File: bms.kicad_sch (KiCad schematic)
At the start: 146 parts, among them J1 Conn_01x08, Q1 DMZ6012E, Q2 DMZ6012E, Q5 BSS123, U8 XC6206P332MR, U9 2SC2383_C41375137

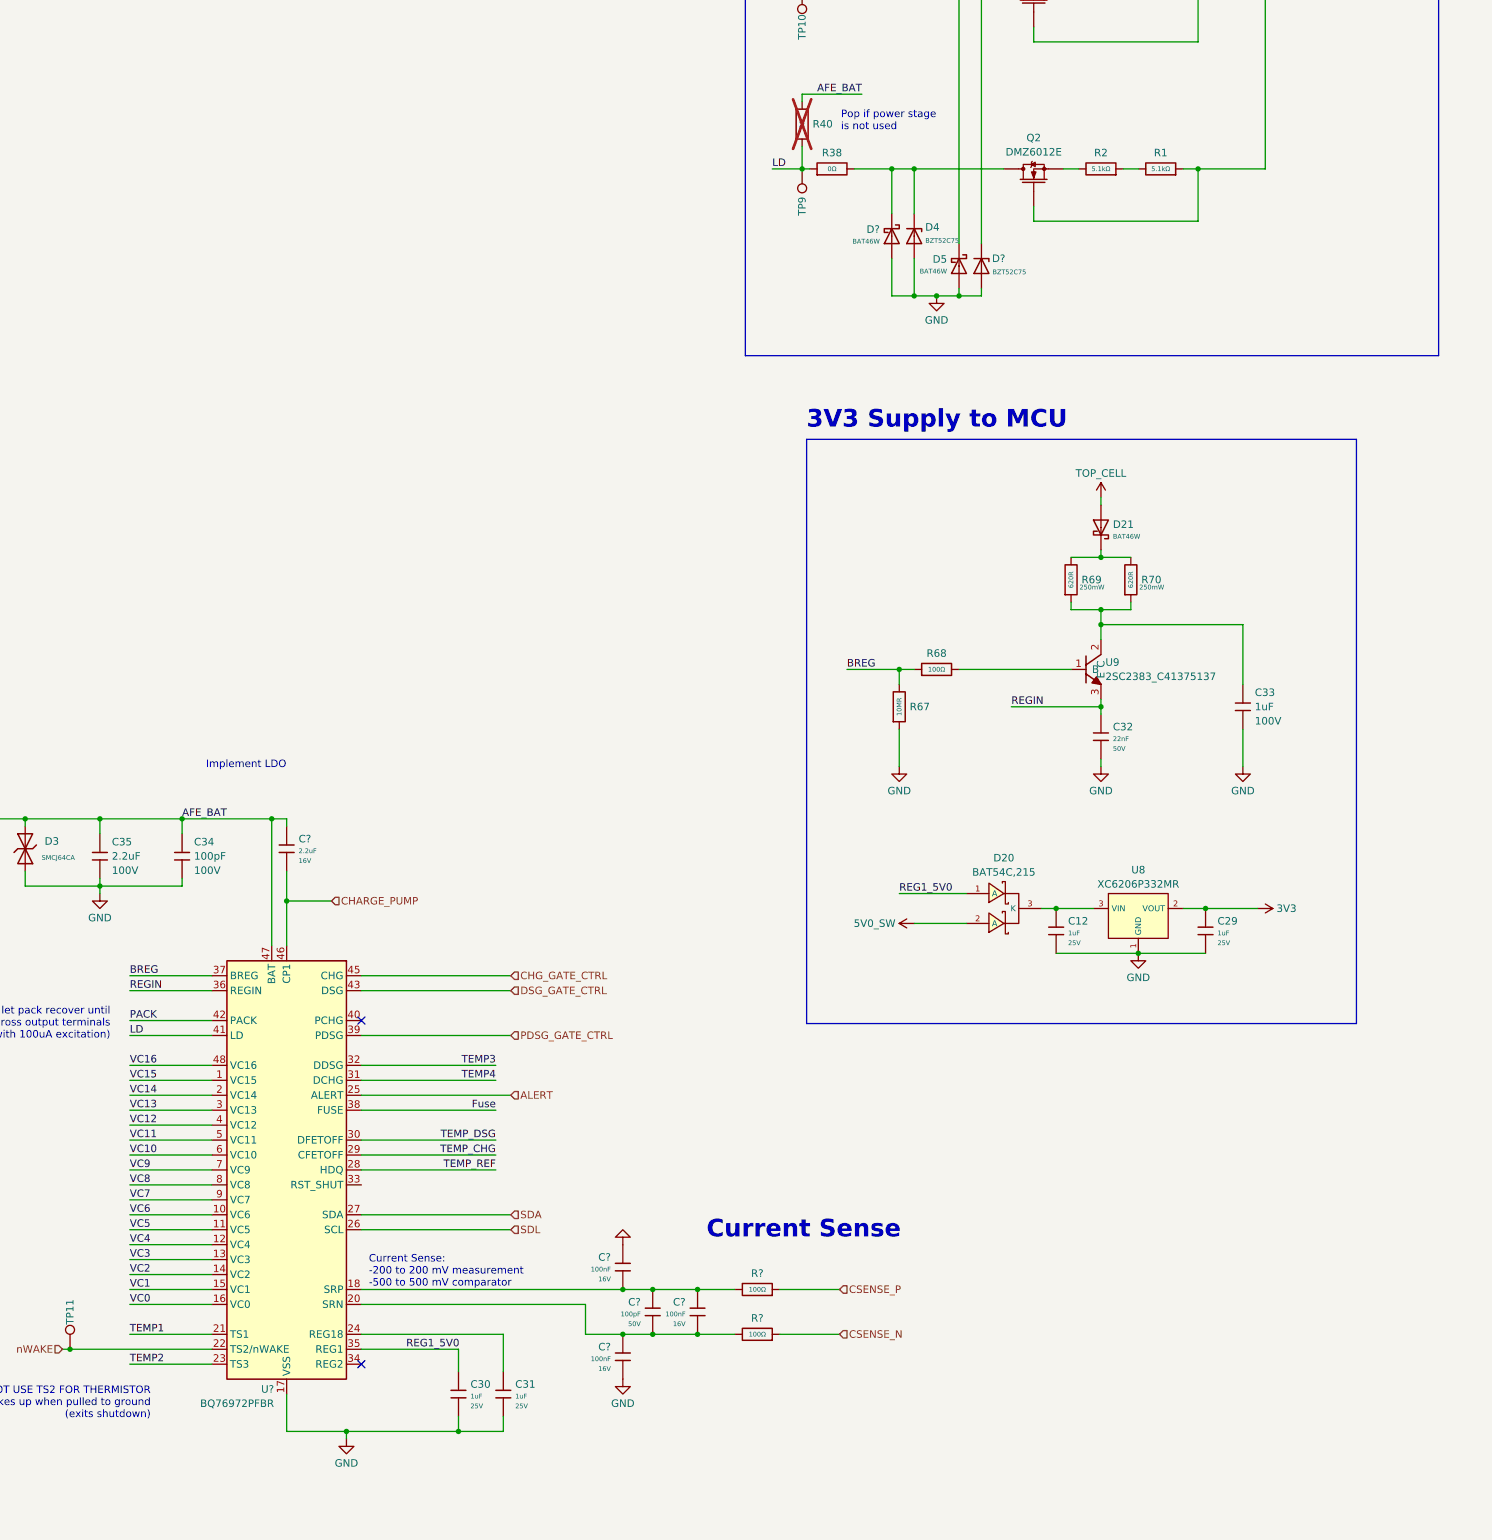
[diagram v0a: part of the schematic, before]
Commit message: Revert "added precharge circuit, filled in placeholder parts"
This reverts commit caa5444a50fe9d2ccb2e95970e40619801e9f697.
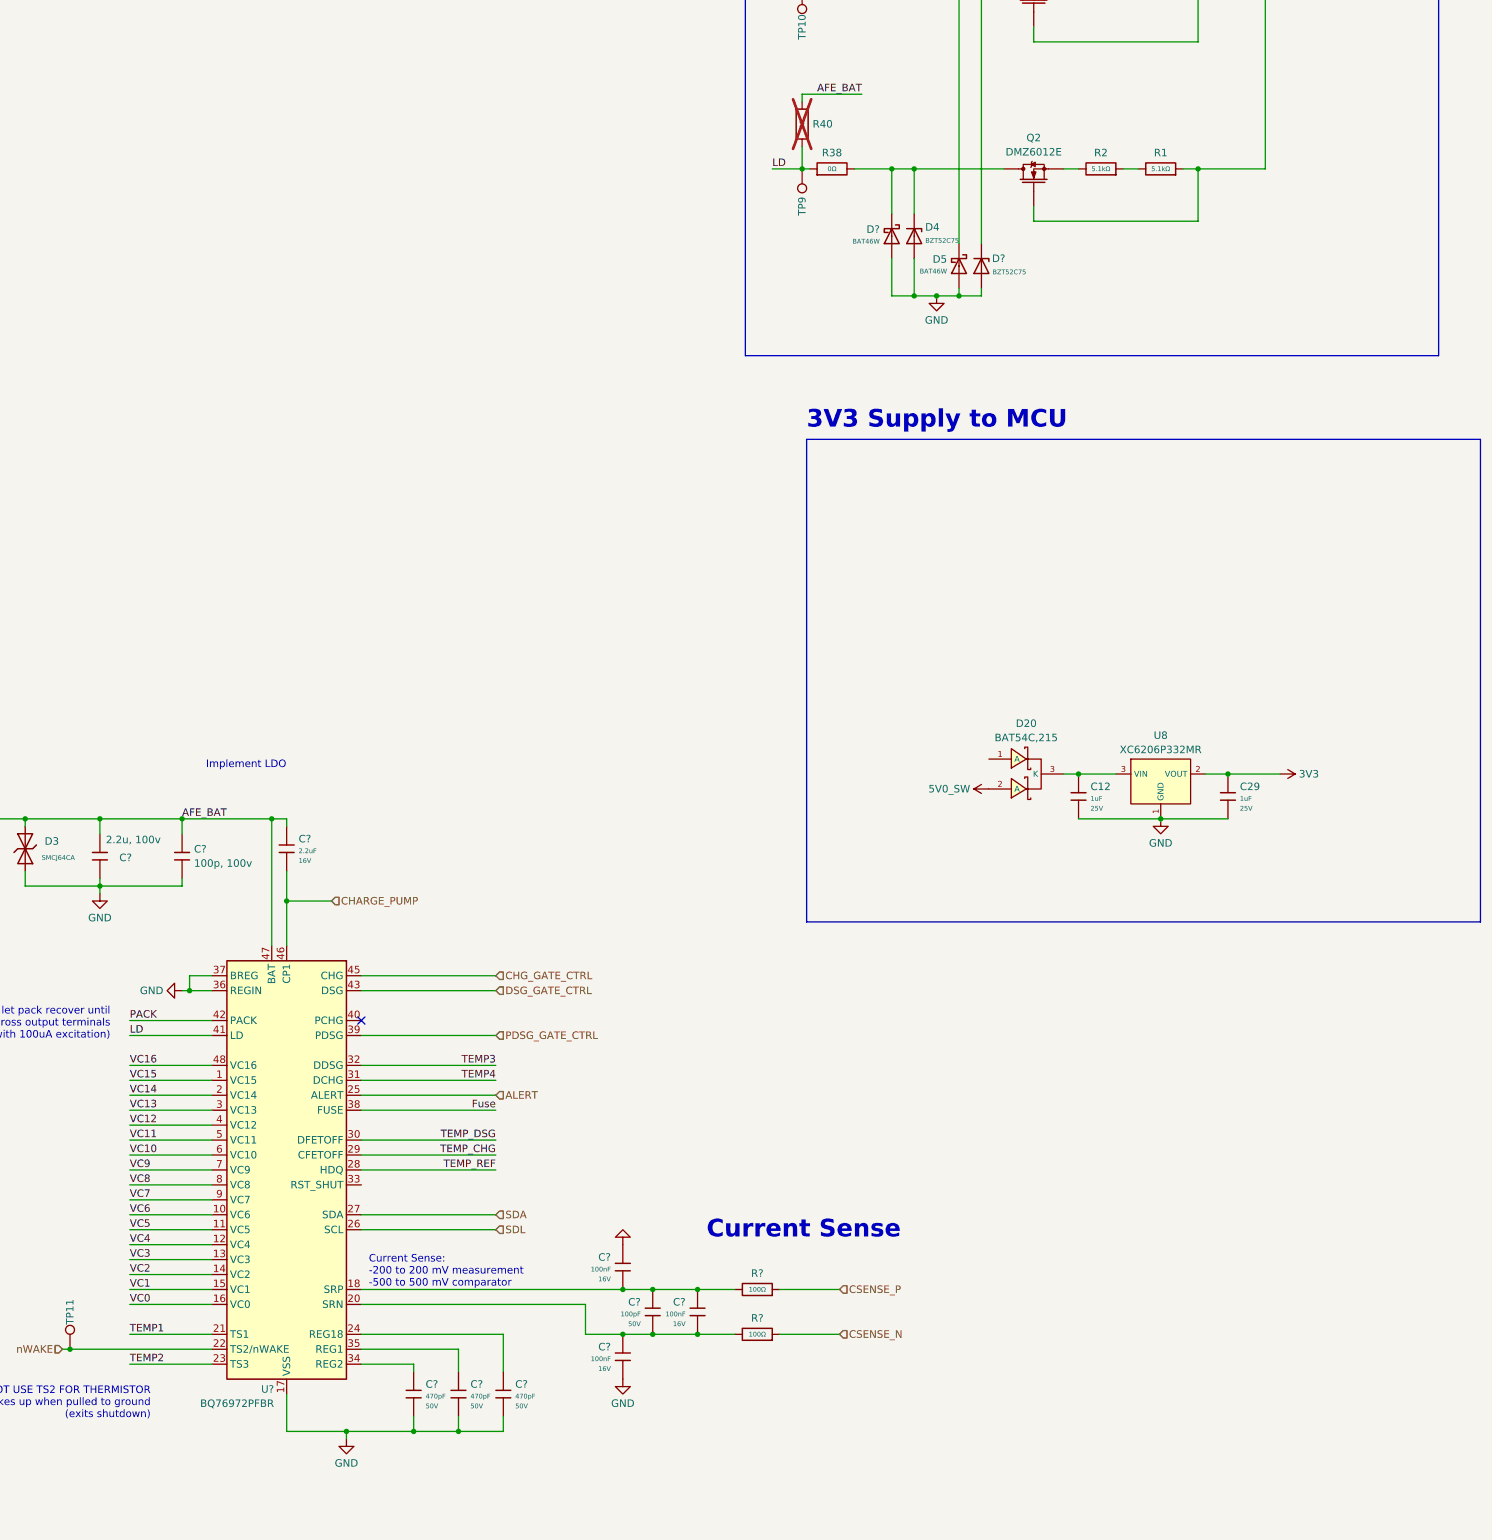
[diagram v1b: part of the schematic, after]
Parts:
- removed C30, C31: 1uF, PCM_JLCPCB:C_0402, symbol PCM_JLCPCB-Capacitors:0402,1uF
- removed C32: 22nF, PCM_JLCPCB:C_0402, symbol PCM_JLCPCB-Capacitors:0402,22nF
- removed C33: 1uF, PCM_JLCPCB:C_0805, symbol ct_lib:CC0805KKX7R0BB105
- removed C34: 100pF, PCM_JLCPCB:C_0603, symbol ct_lib:CC0603JRNPO0BN101
- removed C35: 2.2uF, PCM_JLCPCB:C_1206, symbol ct_lib:CC1206KKX7R0BB225
- removed D21: BAT46W, PCM_JLCPCB:D_SOD-123, symbol PCM_JLCPCB-Diodes:Schottky,BAT46W
- removed R67: 10MR, PCM_JLCPCB:R_0402, symbol ct_lib:RC0402JR-0710ML
- removed R68: 100Ω, PCM_JLCPCB:R_0402, symbol PCM_JLCPCB-Resistors:0402,100Ω
- removed R69, R70: 620R, PCM_JLCPCB:R_1206, symbol ct_lib:1206W4F6200T5E
- removed U9: 2SC2383_C41375137, Package_TO_SOT_SMD:SOT-89-3, symbol JLCImport:2SC2383_C41375137
- added C? (x3): 470pF, PCM_JLCPCB:C_0402, symbol PCM_JLCPCB-Capacitors:0402,470pF
- added C?: 100p, 100v, symbol ct_lib:C
- added C?: 2.2u, 100v, symbol ct_lib:C
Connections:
- net BREG is gone; now on net GND: U?.37 (BREG)
- net REGIN is gone; now on net GND: U?.36 (REGIN)
- net AFE_BAT: now also C?.1, C?.1
- net GND: now also C?.2, C?.2, C?.2, C?.2, C?.2
- net at U?.24 (REG18): now also C?.1
- net at U?.34 (REG2): now also C?.1
- net REG1_5V0: no longer names the net of D20.1 (A)
- net REG1_5V0: no longer U?.35 (REG1)
- new net: C?.1, U?.35 (REG1)
- no-connect marks 2 -> 1
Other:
- note removed: "Pop if power stage is not used"
- moved on the sheet: C12, C29, D20, U8
